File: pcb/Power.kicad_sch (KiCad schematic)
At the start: 12 parts, among them U4 LD39050PU33R, U5 TLV61048, U6 LDK320AM120R

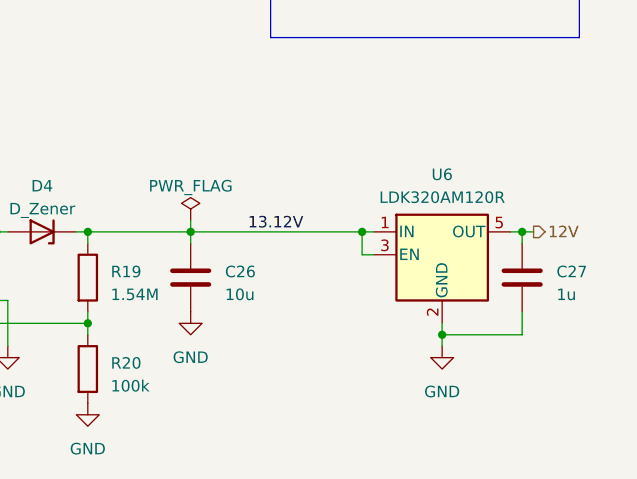
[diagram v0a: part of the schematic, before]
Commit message: Updated PCB
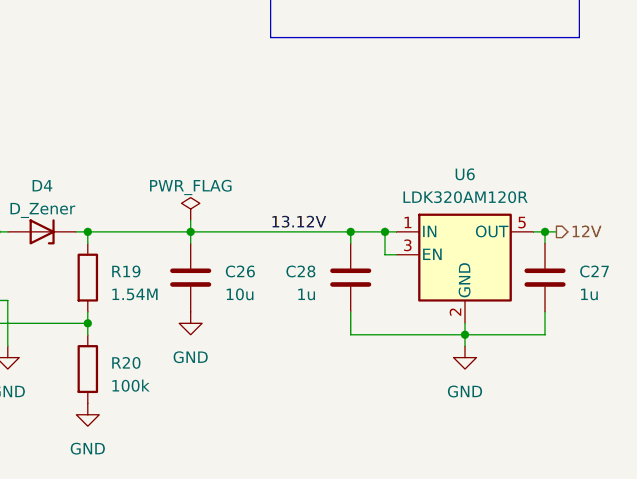
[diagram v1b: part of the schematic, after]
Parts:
- added C28: 1u, Capacitor_SMD:C_0603_1608Metric, symbol Device:C
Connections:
- net 13.12V: now also C28.1
- net GND: now also C28.2
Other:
- moved on the sheet: C27, U6
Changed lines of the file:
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@@
   (junction (at 106.68 76.2) (diameter 0) (color 0 0 0 0)
   )
+  (junction (at 172.72 116.84) (diameter 0) (color 0 0 0 0)
+  )
   (junction (at 106.68 73.66) (diameter 0) (color 0 0 0 0)
   )
-  (junction (at 182.88 128.27) (diameter 0) (color 0 0 0 0)
-  )
-  (junction (at 173.99 116.84) (diameter 0) (color 0 0 0 0)
+  (junction (at 185.42 128.27) (diameter 0) (color 0 0 0 0)
+  )
+  (junction (at 176.53 116.84) (diameter 0) (color 0 0 0 0)
   )
   (junction (at 123.19 88.9) (diameter 0) (color 0 0 0 0)
@@
   (junction (at 113.03 121.92) (diameter 0) (color 0 0 0 0)
   )
-  (junction (at 191.77 116.84) (diameter 0) (color 0 0 0 0)
+  (junction (at 194.31 116.84) (diameter 0) (color 0 0 0 0)
   )
   (junction (at 143.51 127) (diameter 0) (color 0 0 0 0)
@@
   )
   (no_connect (at 133.35 78.74))
-  (wire (pts (xy 191.77 116.84) (xy 190.5 116.84))
-    (stroke (width 0) (type default))
-  )
-  (wire (pts (xy 191.77 125.73) (xy 191.77 128.27))
+  (wire (pts (xy 194.31 116.84) (xy 193.04 116.84))
+    (stroke (width 0) (type default))
+  )
+  (wire (pts (xy 172.72 116.84) (xy 176.53 116.84))
+    (stroke (width 0) (type default))
+  )
+  (wire (pts (xy 194.31 125.73) (xy 194.31 128.27))
     (stroke (width 0) (type default))
   )
@@
     (stroke (width 0) (type default))
   )
-  (wire (pts (xy 191.77 116.84) (xy 193.04 116.84))
+  (wire (pts (xy 194.31 116.84) (xy 195.58 116.84))
     (stroke (width 0) (type default))
   )
@@
     (stroke (width 0) (type default))
   )
-  (wire (pts (xy 175.26 119.38) (xy 173.99 119.38))
-    (stroke (width 0) (type default))
-  )
-  (wire (pts (xy 191.77 118.11) (xy 191.77 116.84))
+  (wire (pts (xy 177.8 119.38) (xy 176.53 119.38))
+    (stroke (width 0) (type default))
+  )
+  (wire (pts (xy 194.31 118.11) (xy 194.31 116.84))
     (stroke (width 0) (type default))
   )
@@
     (stroke (width 0) (type default))
   )
-  (wire (pts (xy 182.88 129.54) (xy 182.88 128.27))
+  (wire (pts (xy 185.42 129.54) (xy 185.42 128.27))
     (stroke (width 0) (type default))
   )
@@
     (stroke (width 0) (type default))
   )
+  (wire (pts (xy 172.72 125.73) (xy 172.72 128.27))
+    (stroke (width 0) (type default))
+  )
   (wire (pts (xy 114.3 124.46) (xy 110.49 124.46))
     (stroke (width 0) (type default))
@@
     (stroke (width 0) (type default))
   )
-  (wire (pts (xy 154.94 116.84) (xy 173.99 116.84))
+  (wire (pts (xy 154.94 116.84) (xy 172.72 116.84))
+    (stroke (width 0) (type default))
+  )
+  (wire (pts (xy 172.72 128.27) (xy 185.42 128.27))
     (stroke (width 0) (type default))
   )
@@
     (stroke (width 0) (type default))
   )
-  (wire (pts (xy 182.88 128.27) (xy 182.88 127))
+  (wire (pts (xy 185.42 128.27) (xy 185.42 127))
     (stroke (width 0) (type default))
   )
@@
     (stroke (width 0) (type default))
   )
-  (wire (pts (xy 173.99 119.38) (xy 173.99 116.84))
-    (stroke (width 0) (type default))
-  )
-  (wire (pts (xy 182.88 128.27) (xy 191.77 128.27))
-    (stroke (width 0) (type default))
-  )
-  (wire (pts (xy 173.99 116.84) (xy 175.26 116.84))
+  (wire (pts (xy 176.53 119.38) (xy 176.53 116.84))
+    (stroke (width 0) (type default))
+  )
+  (wire (pts (xy 185.42 128.27) (xy 194.31 128.27))
+    (stroke (width 0) (type default))
+  )
+  (wire (pts (xy 176.53 116.84) (xy 177.8 116.84))
     (stroke (width 0) (type default))
   )
@@
   )
   (wire (pts (xy 113.03 121.92) (xy 113.03 116.84))
+    (stroke (width 0) (type default))
+  )
+  (wire (pts (xy 172.72 116.84) (xy 172.72 118.11))
     (stroke (width 0) (type default))
   )
@@
     (effects (font (size 1.27 1.27)) (justify left top))
   )
-  (label "13.12V" (at 161.29 116.84 0) (fields_autoplaced)
+  (label "13.12V" (at 163.83 116.84 0) (fields_autoplaced)
     (effects (font (size 1.27 1.27)) (justify left bottom))
   )
-  (hierarchical_label "12V" (shape output) (at 193.04 116.84 0) (fields_autoplaced)
+  (hierarchical_label "12V" (shape output) (at 195.58 116.84 0) (fields_autoplaced)
     (effects (font (size 1.27 1.27)) (justify left))
   )
@@
     )
   )
-  (symbol (lib_id "Signal Generator Components:LDK320AM120R") (at 182.88 119.38 0) (unit 1)
-    (in_bom yes) (on_board yes) (dnp no) (fields_autoplaced)
-    (property "Reference" "U6" (at 182.88 110.49 0)
-      (effects (font (size 1.27 1.27)))
-    )
-    (property "Value" "LDK320AM120R" (at 182.88 113.03 0)
-      (effects (font (size 1.27 1.27)))
-    )
-    (property "Footprint" "Signal Generator Components:LDK320AM120R" (at 177.8 110.49 0)
-      (effects (font (size 1.27 1.27)) hide)
-    )
-    (property "Datasheet" "" (at 182.88 119.38 0)
-      (effects (font (size 1.27 1.27)) hide)
-    )
-    (property "PN" "LDK320AM120R" (at 182.88 119.38 0)
+  (symbol (lib_id "Signal Generator Components:LDK320AM120R") (at 185.42 119.38 0) (unit 1)
+    (in_bom yes) (on_board yes) (dnp no) (fields_autoplaced)
+    (property "Reference" "U6" (at 185.42 110.49 0)
+      (effects (font (size 1.27 1.27)))
+    )
+    (property "Value" "LDK320AM120R" (at 185.42 113.03 0)
+      (effects (font (size 1.27 1.27)))
+    )
+    (property "Footprint" "Signal Generator Components:LDK320AM120R" (at 180.34 110.49 0)
+      (effects (font (size 1.27 1.27)) hide)
+    )
+    (property "Datasheet" "" (at 185.42 119.38 0)
+      (effects (font (size 1.27 1.27)) hide)
+    )
+    (property "PN" "LDK320AM120R" (at 185.42 119.38 0)
       (effects (font (size 1.27 1.27)) hide)
     )
@@
     )
   )
-  (symbol (lib_id "Device:C") (at 191.77 121.92 0) (unit 1)
-    (in_bom yes) (on_board yes) (dnp no) (fields_autoplaced)
-    (property "Reference" "C27" (at 195.58 121.285 0)
-      (effects (font (size 1.27 1.27)) (justify left))
-    )
-    (property "Value" "1u" (at 195.58 123.825 0)
-      (effects (font (size 1.27 1.27)) (justify left))
-    )
-    (property "Footprint" "Capacitor_SMD:C_0603_1608Metric" (at 192.7352 125.73 0)
-      (effects (font (size 1.27 1.27)) hide)
-    )
-    (property "Datasheet" "~" (at 191.77 121.92 0)
-      (effects (font (size 1.27 1.27)) hide)
-    )
-    (property "PN" "GCM188R71C105KA64D" (at 191.77 121.92 0)
+  (symbol (lib_id "Device:C") (at 194.31 121.92 0) (unit 1)
+    (in_bom yes) (on_board yes) (dnp no) (fields_autoplaced)
+    (property "Reference" "C27" (at 198.12 121.285 0)
+      (effects (font (size 1.27 1.27)) (justify left))
+    )
+    (property "Value" "1u" (at 198.12 123.825 0)
+      (effects (font (size 1.27 1.27)) (justify left))
+    )
+    (property "Footprint" "Capacitor_SMD:C_0603_1608Metric" (at 195.2752 125.73 0)
+      (effects (font (size 1.27 1.27)) hide)
+    )
+    (property "Datasheet" "~" (at 194.31 121.92 0)
+      (effects (font (size 1.27 1.27)) hide)
+    )
+    (property "PN" "GCM188R71C105KA64D" (at 194.31 121.92 0)
       (effects (font (size 1.27 1.27)) hide)
     )
@@
         (path "/f6255c48-6253-4c69-a6db-1ceaf4eff04d/755a5482-c972-48ba-877b-a349f74d45fc"
           (reference "#PWR0133") (unit 1)
+        )
+      )
+    )
+  )
+  (symbol (lib_id "Device:C") (at 172.72 121.92 0) (mirror y) (unit 1)
+    (in_bom yes) (on_board yes) (dnp no)
+    (property "Reference" "C28" (at 168.91 121.285 0)
+      (effects (font (size 1.27 1.27)) (justify left))
+    )
+    (property "Value" "1u" (at 168.91 123.825 0)
+      (effects (font (size 1.27 1.27)) (justify left))
+    )
+    (property "Footprint" "Capacitor_SMD:C_0603_1608Metric" (at 171.7548 125.73 0)
+      (effects (font (size 1.27 1.27)) hide)
+    )
+    (property "Datasheet" "~" (at 172.72 121.92 0)
+      (effects (font (size 1.27 1.27)) hide)
+    )
+    (property "PN" "GCM188R71C105KA64D" (at 172.72 121.92 0)
+      (effects (font (size 1.27 1.27)) hide)
+    )
+    (pin "1")
+    (pin "2")
+    (instances
+      (project "Signal Generator"
+        (path "/f6255c48-6253-4c69-a6db-1ceaf4eff04d/755a5482-c972-48ba-877b-a349f74d45fc"
+          (reference "C28") (unit 1)
         )
       )
@@
     )
   )
-  (symbol (lib_id "power:GND") (at 182.88 129.54 0) (unit 1)
-    (in_bom yes) (on_board yes) (dnp no) (fields_autoplaced)
-    (property "Reference" "#PWR010" (at 182.88 135.89 0)
-      (effects (font (size 1.27 1.27)) hide)
-    )
-    (property "Value" "GND" (at 182.88 134.62 0)
-      (effects (font (size 1.27 1.27)))
-    )
-    (property "Footprint" "" (at 182.88 129.54 0)
-      (effects (font (size 1.27 1.27)) hide)
-    )
-    (property "Datasheet" "" (at 182.88 129.54 0)
-      (effects (font (size 1.27 1.27)) hide)
-    )
+  (symbol (lib_id "power:GND") (at 185.42 129.54 0) (unit 1)
+    (in_bom yes) (on_board yes) (dnp no) (fields_autoplaced)
+    (property "Reference" "#PWR010" (at 185.42 135.89 0)
+      (effects (font (size 1.27 1.27)) hide)
+    )
+    (property "Value" "GND" (at 185.42 134.62 0)
+      (effects (font (size 1.27 1.27)))
+    )
+    (property "Footprint" "" (at 185.42 129.54 0)
+      (effects (font (size 1.27 1.27)) hide)
+    )
+    (property "Datasheet" "" (at 185.42 129.54 0)
+      (effects (font (size 1.27 1.27)) hide)
+    )
